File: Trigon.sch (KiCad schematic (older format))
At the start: 1 part

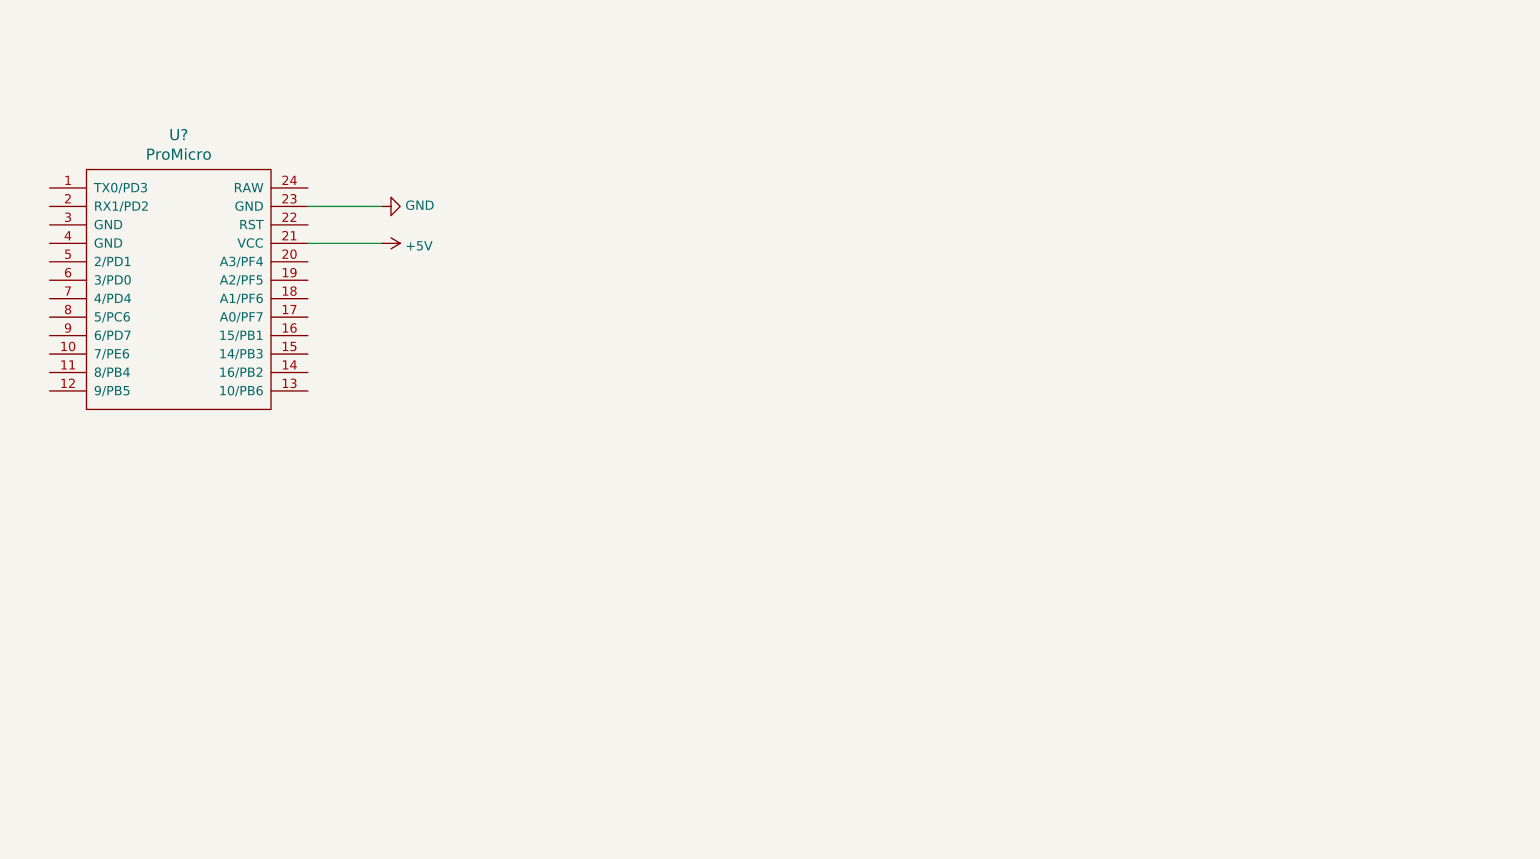
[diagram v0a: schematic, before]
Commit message: Fully laid out board
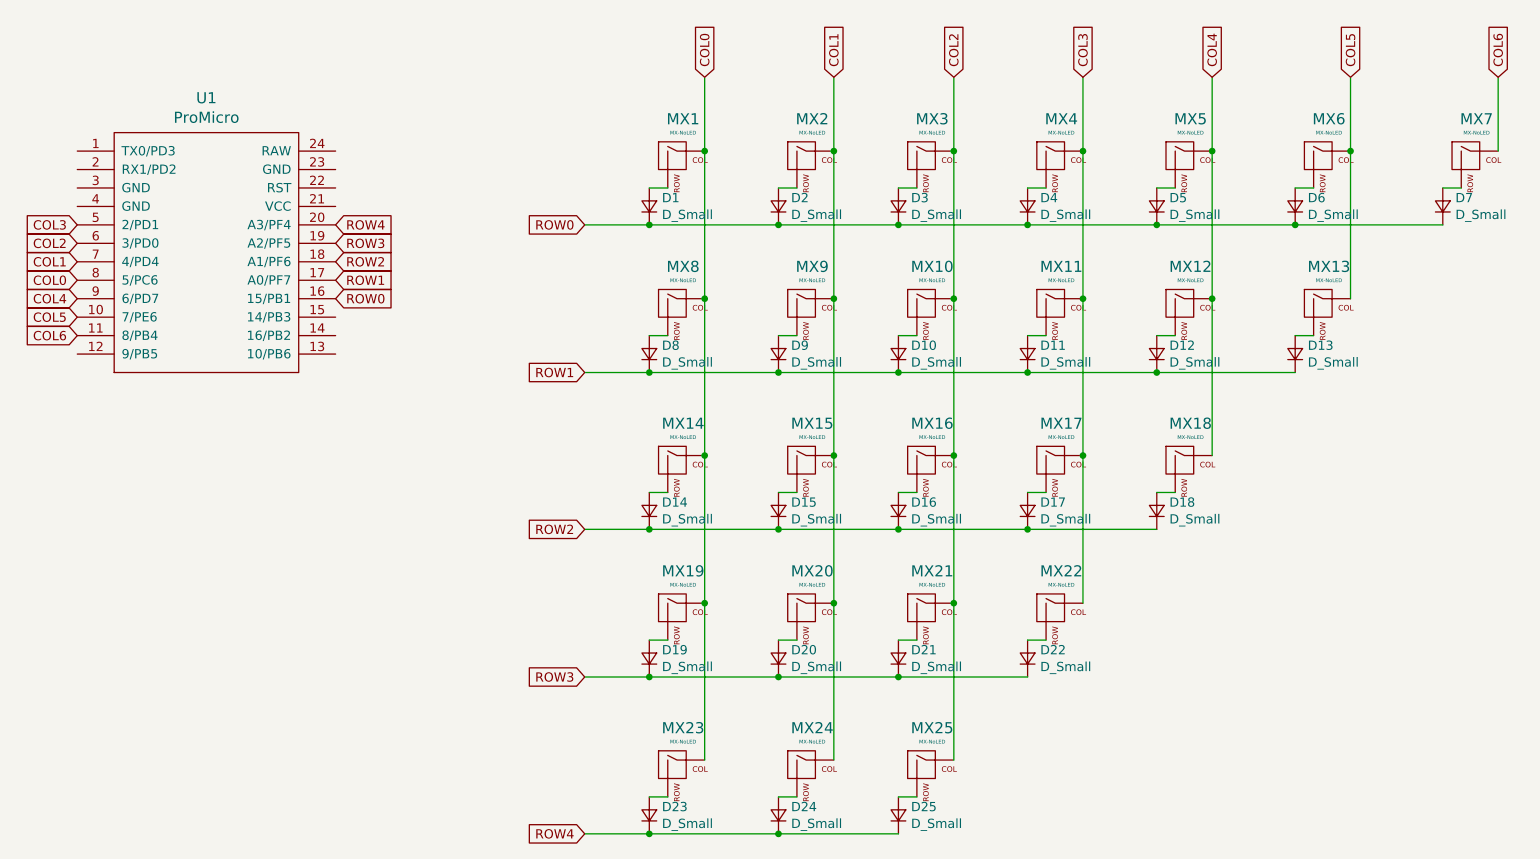
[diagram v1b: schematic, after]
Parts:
- removed U?: ProMicro, symbol keebio:ProMicro
- added D1, D10, D11, D12, D13, D14, D15, D16, D17, D18, D19, D2, D20, D21, D22, D23, D24, D25, D3, D4, D5, D6, D7, D8, D9: D_Small, Keebio-Parts:Diode, symbol Device:D_Small
- added MX1, MX10, MX11, MX12, MX13, MX14, MX15, MX16, MX17, MX18, MX19, MX2, MX20, MX21, MX22, MX23, MX24, MX25, MX3, MX4, MX5, MX6, MX7, MX8, MX9: MX-NoLED, MX_Alps_Hybrid:MX-1U-NoLED, symbol MX_Alps_Hybrid:MX-NoLED
- added U1: ProMicro, Keebio-Parts:ArduinoProMicro-ZigZag, symbol keebio:ProMicro
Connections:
- new net: D1.2 (A), MX1.2 (ROW)
- new net: D2.2 (A), MX2.2 (ROW)
- new net: D3.2 (A), MX3.2 (ROW)
- new net: D4.2 (A), MX4.2 (ROW)
- new net: D5.2 (A), MX5.2 (ROW)
- new net: D6.2 (A), MX6.2 (ROW)
- new net: D7.2 (A), MX7.2 (ROW)
- new net: D8.2 (A), MX8.2 (ROW)
- new net: D9.2 (A), MX9.2 (ROW)
- new net: D10.2 (A), MX10.2 (ROW)
- new net: D11.2 (A), MX11.2 (ROW)
- new net: D12.2 (A), MX12.2 (ROW)
- new net: D13.2 (A), MX13.2 (ROW)
- new net: D14.2 (A), MX14.2 (ROW)
- new net: D15.2 (A), MX15.2 (ROW)
- new net: D16.2 (A), MX16.2 (ROW)
- new net: D17.2 (A), MX17.2 (ROW)
- new net: D18.2 (A), MX18.2 (ROW)
- new net: D19.2 (A), MX19.2 (ROW)
- new net: D20.2 (A), MX20.2 (ROW)
- new net: D21.2 (A), MX21.2 (ROW)
- new net: D22.2 (A), MX22.2 (ROW)
- new net: D23.2 (A), MX23.2 (ROW)
- new net: D24.2 (A), MX24.2 (ROW)
- new net: D25.2 (A), MX25.2 (ROW)
- new net COL0: MX1.1 (COL), MX14.1 (COL), MX19.1 (COL), MX23.1 (COL), MX8.1 (COL), U1.8 (5/PC6)
- new net COL1: MX15.1 (COL), MX2.1 (COL), MX20.1 (COL), MX24.1 (COL), MX9.1 (COL), U1.7 (4/PD4)
- new net COL2: MX10.1 (COL), MX16.1 (COL), MX21.1 (COL), MX25.1 (COL), MX3.1 (COL), U1.6 (3/PD0)
- new net COL3: MX11.1 (COL), MX17.1 (COL), MX22.1 (COL), MX4.1 (COL), U1.5 (2/PD1)
- new net COL4: MX12.1 (COL), MX18.1 (COL), MX5.1 (COL), U1.9 (6/PD7)
- new net COL5: MX13.1 (COL), MX6.1 (COL), U1.10 (7/PE6)
- new net COL6: MX7.1 (COL), U1.11 (8/PB4)
- new net ROW0: D1.1 (K), D2.1 (K), D3.1 (K), D4.1 (K), D5.1 (K), D6.1 (K), D7.1 (K), U1.16 (15/PB1)
- new net ROW1: D10.1 (K), D11.1 (K), D12.1 (K), D13.1 (K), D8.1 (K), D9.1 (K), U1.17 (A0/PF7)
- new net ROW2: D14.1 (K), D15.1 (K), D16.1 (K), D17.1 (K), D18.1 (K), U1.18 (A1/PF6)
- new net ROW3: D19.1 (K), D20.1 (K), D21.1 (K), D22.1 (K), U1.19 (A2/PF5)
- new net ROW4: D23.1 (K), D24.1 (K), D25.1 (K), U1.20 (A3/PF4)
